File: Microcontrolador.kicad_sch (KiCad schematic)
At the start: 1 part, among them IC2 R7F125FPL4AFB-C#UA0

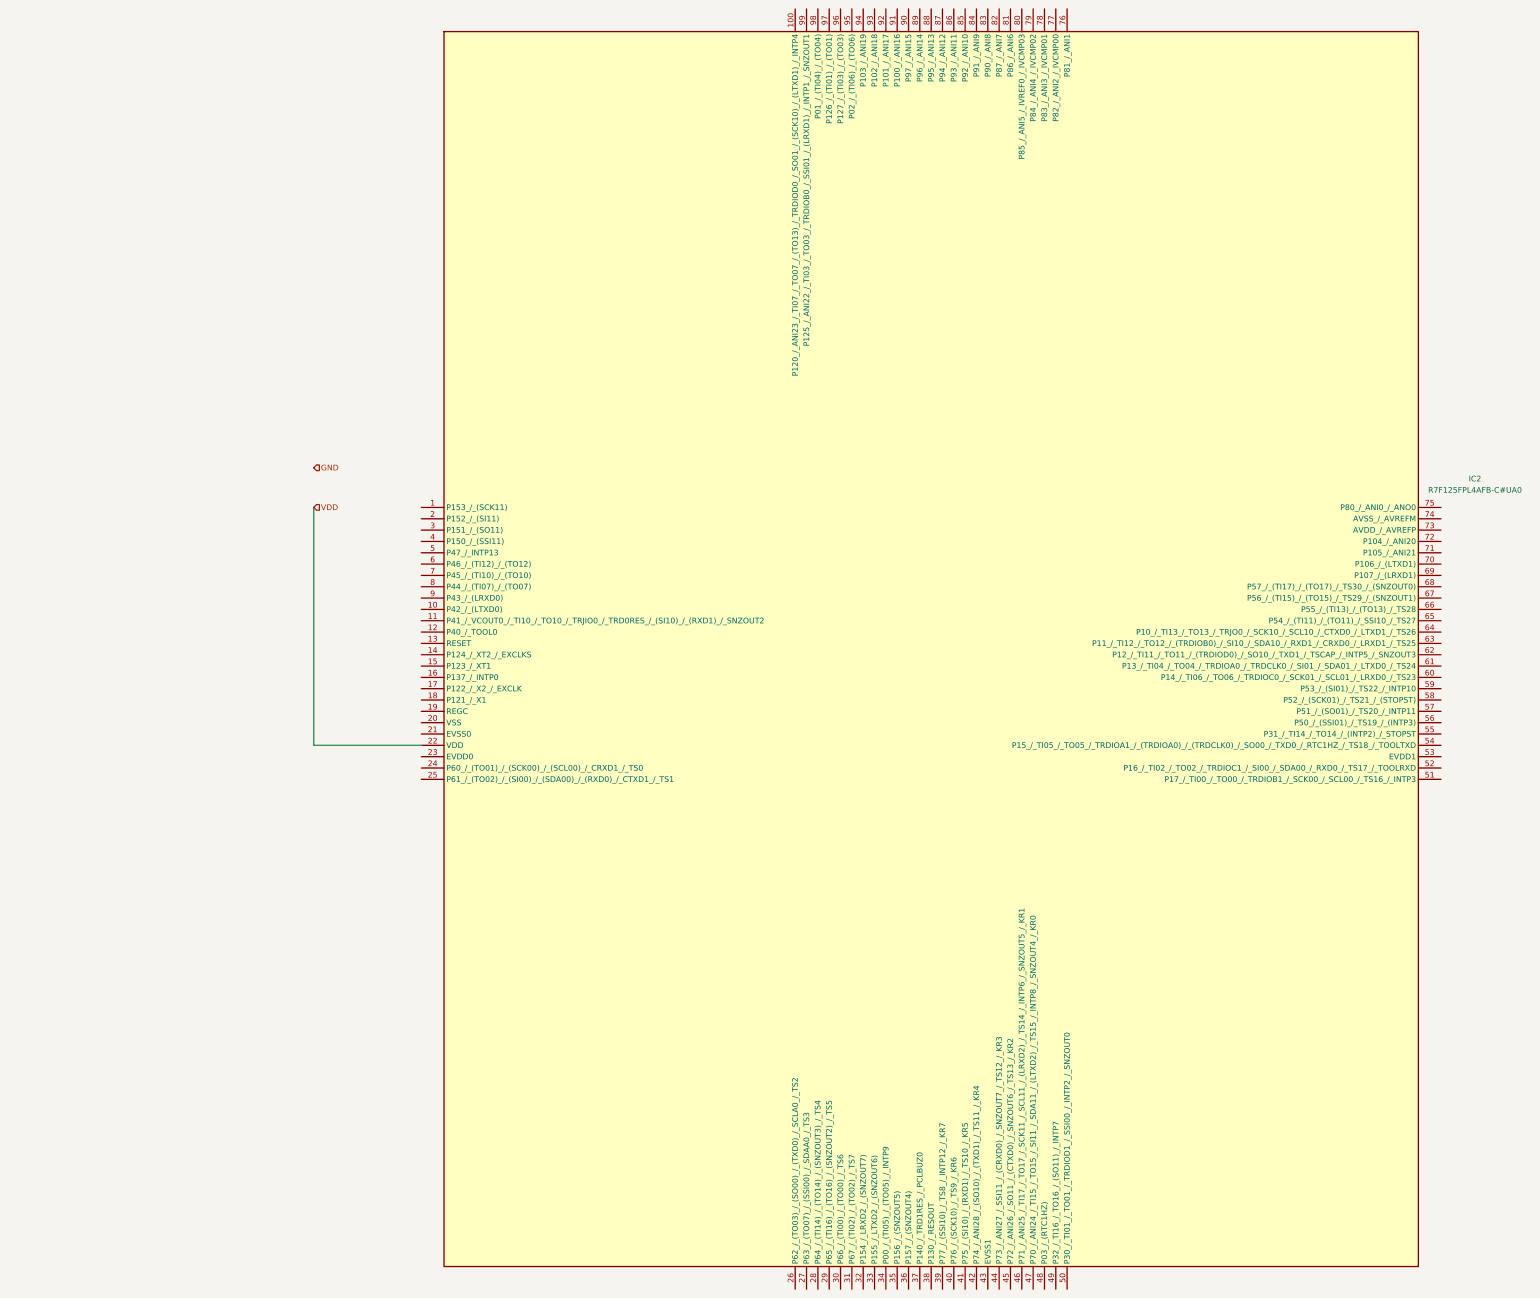
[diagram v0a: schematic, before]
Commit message: Add files via upload
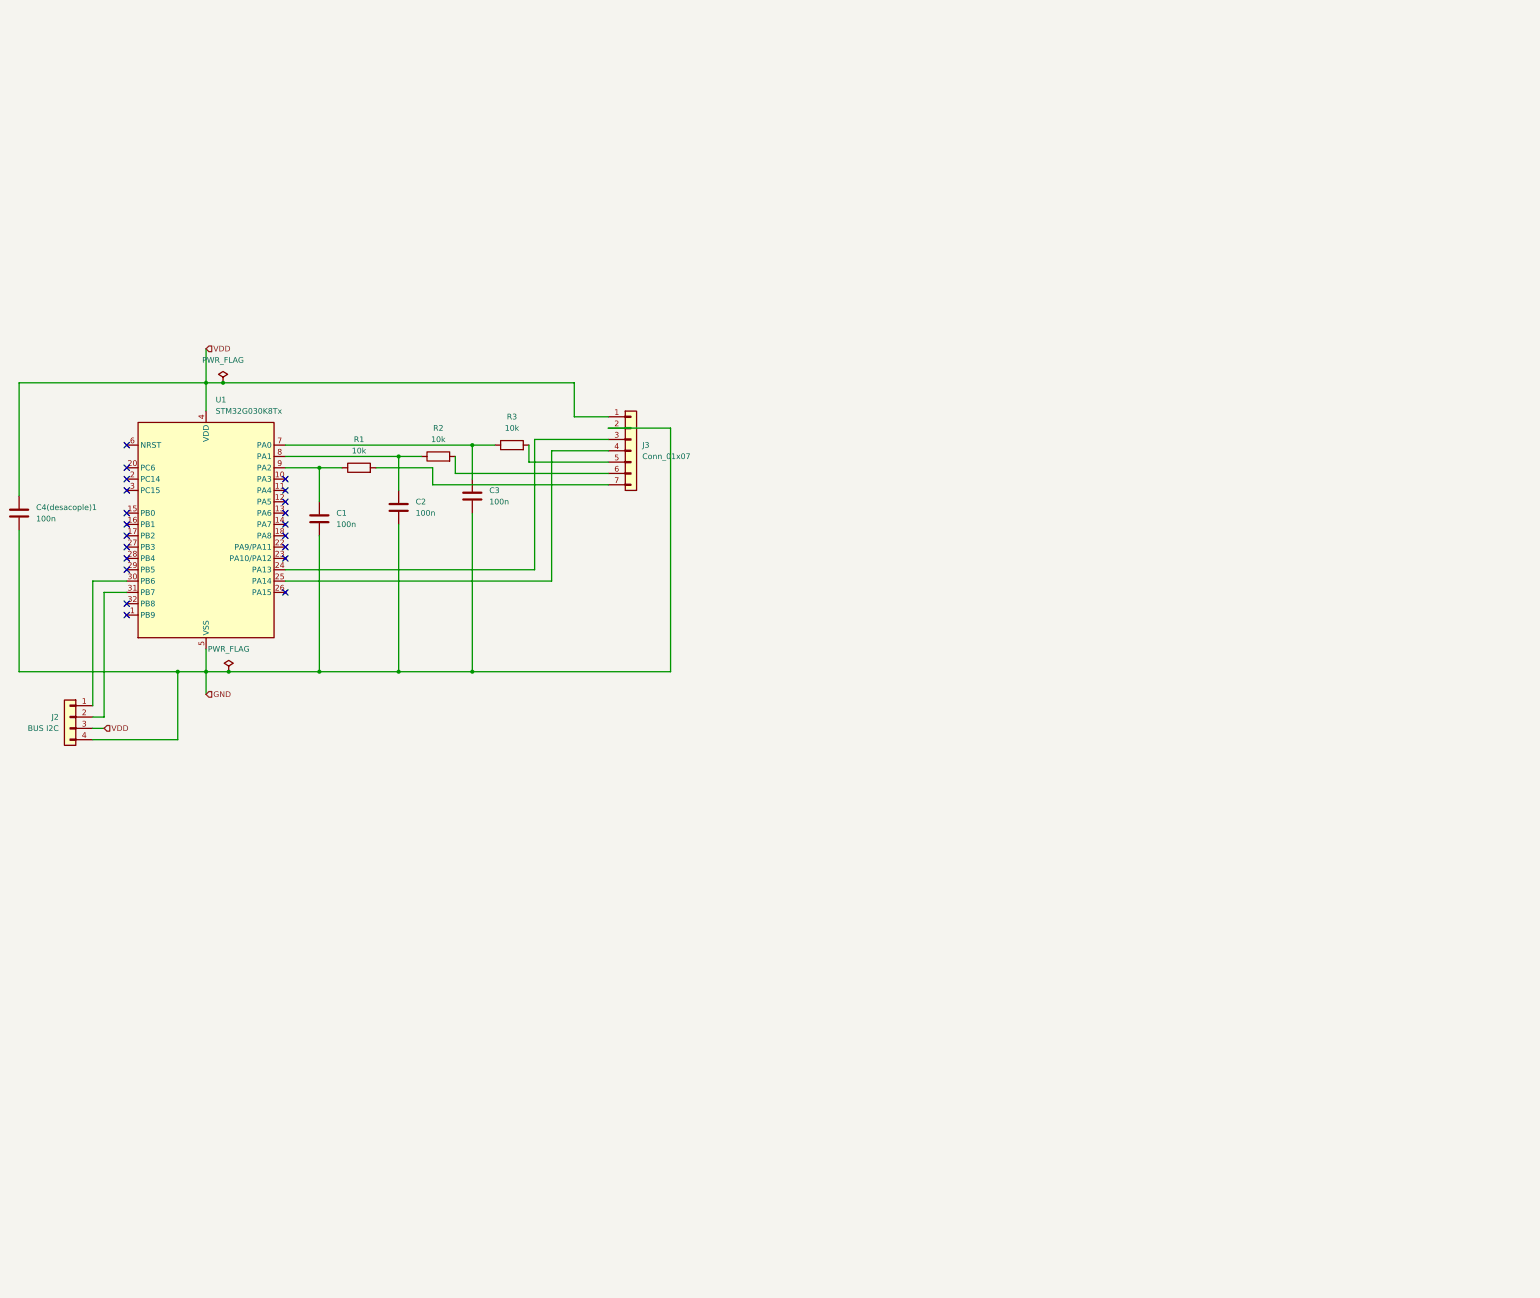
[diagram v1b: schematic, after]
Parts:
- removed IC2: R7F125FPL4AFB-C#UA0, QFP50P1600X1600X160-100N, symbol R7F125FPL4AFB-C#UA0:R7F125FPL4AFB-C#UA0
- added C1, C2, C3, C4(desacople)1: 100n, Capacitor_SMD:C_0805_2012Metric, symbol Device:C
- added J2: BUS I2C, Connector_PinHeader_2.54mm:PinHeader_1x04_P2.54mm_Vertical, symbol Connector_Generic:Conn_01x04
- added J3: Conn_01x07, Connector_PinHeader_2.54mm:PinHeader_1x07_P2.54mm_Horizontal, symbol Connector_Generic:Conn_01x07
- added R1, R2, R3: 10k, Resistor_SMD:R_0805_2012Metric, symbol Device:R
- added U1: STM32G030K8Tx, Package_QFP:LQFP-32_7x7mm_P0.8mm, symbol MCU_ST_STM32G0:STM32G030K8Tx
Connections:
- net GND: now also C1.2, C2.2, C3.2, C4(desacople)1.2, J2.4 (Pin_4), J3.2 (Pin_2), U1.5 (VSS)
- net VDD: now also C4(desacople)1.1, J2.3 (Pin_3), J3.1 (Pin_1), U1.4 (VDD)
- new net: C3.1, R3.1, U1.7 (PA0)
- new net: C2.1, R2.1, U1.8 (PA1)
- new net: J3.6 (Pin_6), R2.2
- new net: C1.1, R1.1, U1.9 (PA2)
- new net: J3.7 (Pin_7), R1.2
- new net: J3.5 (Pin_5), R3.2
- new net: J3.3 (Pin_3), U1.24 (PA13)
- new net: J3.4 (Pin_4), U1.25 (PA14)
- new net: J2.1 (Pin_1), U1.30 (PB6)
- new net: J2.2 (Pin_2), U1.31 (PB7)
- no-connect marks 0 -> 21
